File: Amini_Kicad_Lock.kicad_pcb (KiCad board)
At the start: 2 copper layers, 27.9 x 19.1 mm, 39 parts, among them J1 Conn_01x02, J2 Conn_01x04, J3 MM8130-2600RA2, J4 Conn_01x03_Pin, U1 nRF5340-QKxx, X1 32MHz, X2 32.768kHz

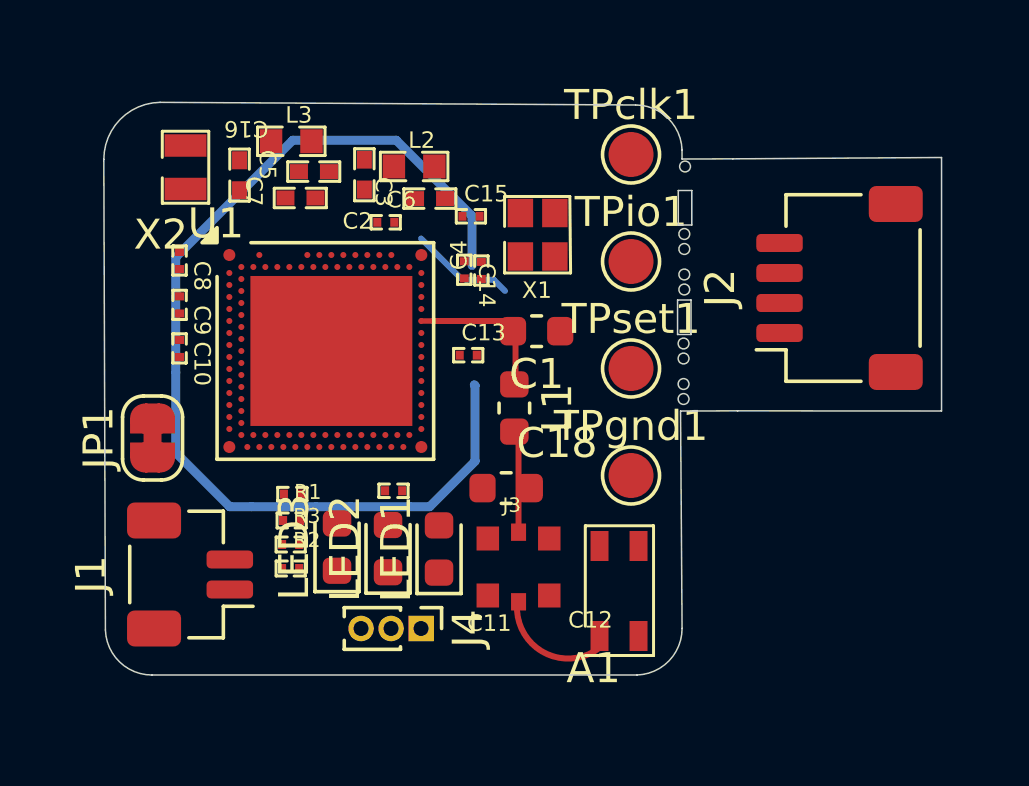
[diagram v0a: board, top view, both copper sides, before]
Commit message: backup mid routing
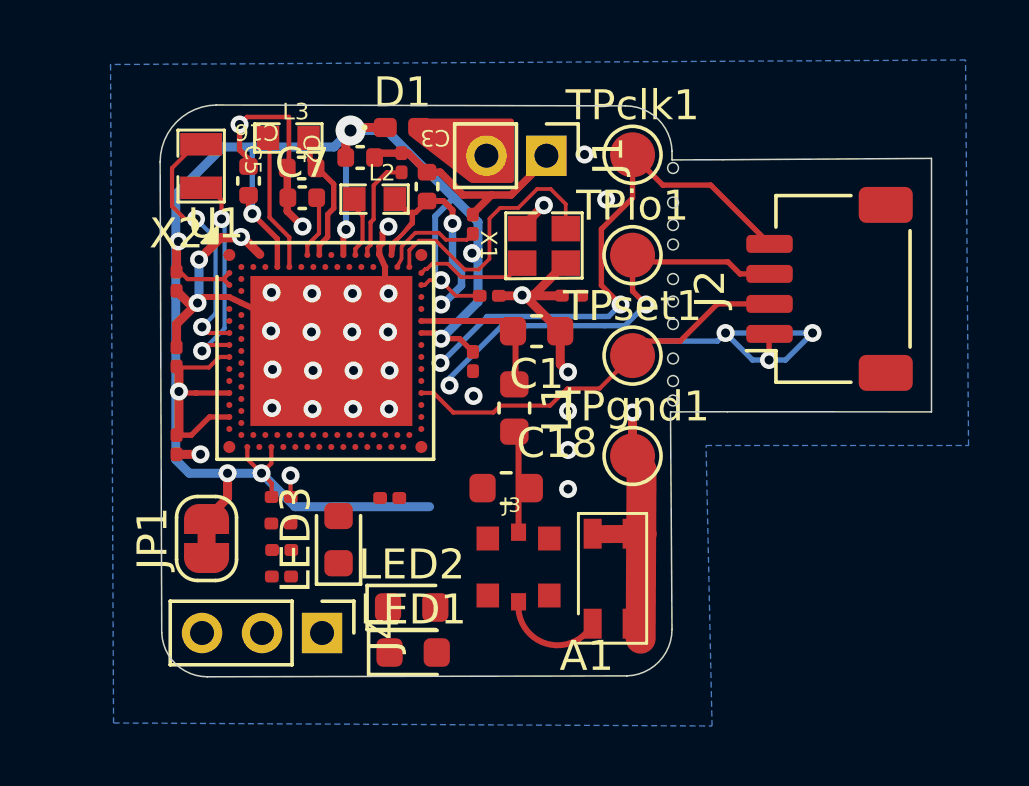
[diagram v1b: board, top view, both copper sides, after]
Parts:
- added D1: D, Diode_SMD:D_0402_1005Metric_Pad0.77x0.64mm_HandSolder, F.Cu at (179.8, 54.4)
- C7: footprint Nordic_Semiconductor:CAPC1005X04L -> Capacitor_SMD:C_0402_1005Metric
- J1: value Conn_01x02 -> Conn_01x02_Pin; footprint Connector_JST:JST_SH_BM02B-SRSS-TB_1x02-1MP_P1.00mm_Vertical -> Connector_PinHeader_2.00mm:PinHeader_1x02_P2.00mm_Vertical
- J4: footprint Connector_PinHeader_1.00mm:PinHeader_1x03_P1.00mm_Vertical -> Connector_PinHeader_2.00mm:PinHeader_1x03_P2.00mm_Vertical
- moved J1 18.3 mm to (184.6, 55.3), turned to -90 degrees
- moved JP1 3.80 mm to (173.2, 68.1)
- moved LED1 3.56 mm to (180.1, 71.9), turned to 0 degrees
- moved C2 3.54 mm to (176.2, 55.1), turned to -90 degrees
- moved C4 3.33 mm to (185.7, 60.0), turned to 180 degrees
- moved J4 3.30 mm to (177.1, 71.2)
- moved C3 3.20 mm to (180.9, 54.2), turned to 180 degrees
- moved C10 3.15 mm to (172.2, 64.7)
- moved X1 2.91 mm to (182.1, 58.3), turned to -90 degrees
- moved C9 2.22 mm to (172.3, 62.3), turned to 90 degrees
- moved C7 2.12 mm to (176.4, 56.7), turned to 0 degrees
- moved LED2 2.11 mm to (180.1, 70.4), turned to 0 degrees
- moved C6 1.87 mm to (179.8, 55.9), turned to 90 degrees
- moved R2 1.83 mm to (175.8, 67.4), turned to 180 degrees
- moved L2 1.71 mm to (179.1, 57.9)
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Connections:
- J1 pad 2: VDD_nRF -> Net-(D1-A)
- U1 pad A25: unconnected-(U1-NC-PadA25) -> GND
- U1 pad B26: unconnected-(U1-NC-PadB26) -> GND
- U1 pad F2: unconnected-(U1-NC-PadF2) -> GND
- U1 pad G1: unconnected-(U1-NC-PadG1) -> GND
- U1 pad H2: unconnected-(U1-NC-PadH2) -> GND
- U1 pad J1: unconnected-(U1-DCCH-PadJ1) -> GND
- X1 pad 4: unconnected-(X1-GND-Pad4) -> GND
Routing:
- net VDD_nRF: track 0.00 -> 71.6 mm, vias 0 -> 10
- net GND: track 0.00 -> 45.2 mm, vias 0 -> 37
- net (no net): track 38.1 -> 0.00 mm
- net /SWDCLK: track 0.00 -> 18.3 mm, vias 0 -> 2
- net /SWDIO: track 0.00 -> 14.5 mm, vias 0 -> 2
- net /~{RESET}: track 0.00 -> 13.4 mm
- net Net-(U1-XL1/P0.00): track 0.00 -> 8.59 mm, vias 0 -> 2
- net /XC2: track 0.00 -> 8.22 mm
- net Net-(U1-XL2/P0.01): track 0.00 -> 6.96 mm, vias 0 -> 2
- net Net-(U1-DECR): track 0.00 -> 6.70 mm, vias 0 -> 2
- net Net-(U1-DCCD): track 0.00 -> 4.82 mm
- net Net-(U1-DECD): track 0.00 -> 4.68 mm
- net /XC1: track 0.00 -> 3.87 mm
- net Net-(U1-DECN): track 0.00 -> 3.52 mm
- net Net-(U1-DECA): track 0.00 -> 2.10 mm
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- added copper zone on B.Cu, net GND
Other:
- board size 27.9 x 19.1 mm -> 25.7 x 19.1 mm
